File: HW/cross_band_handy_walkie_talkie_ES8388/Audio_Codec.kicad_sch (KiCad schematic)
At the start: 73 parts, among them J3 Screw_Terminal_01x02, J4 Conn_01x06, J5 Screw_Terminal_01x02, J6 AudioJack4_SwitchTR1, J7 SMA, J8 SMA, U5 ES8388, U6 TPA2012D2, U7 SA818S, U8 SA818S

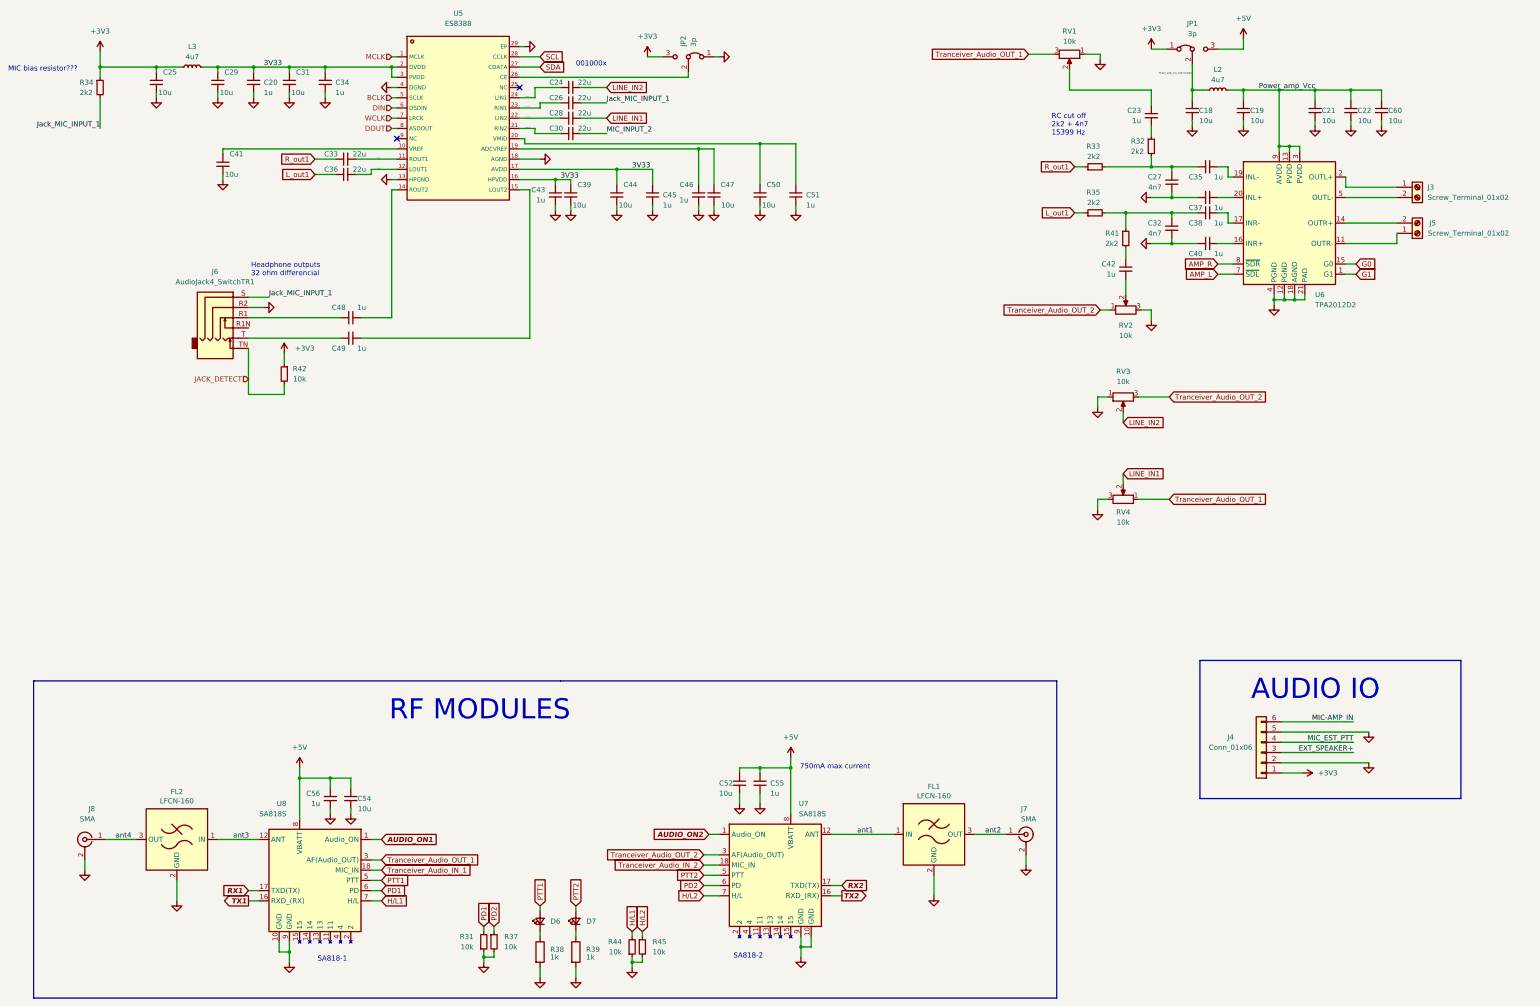
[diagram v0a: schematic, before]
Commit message: r
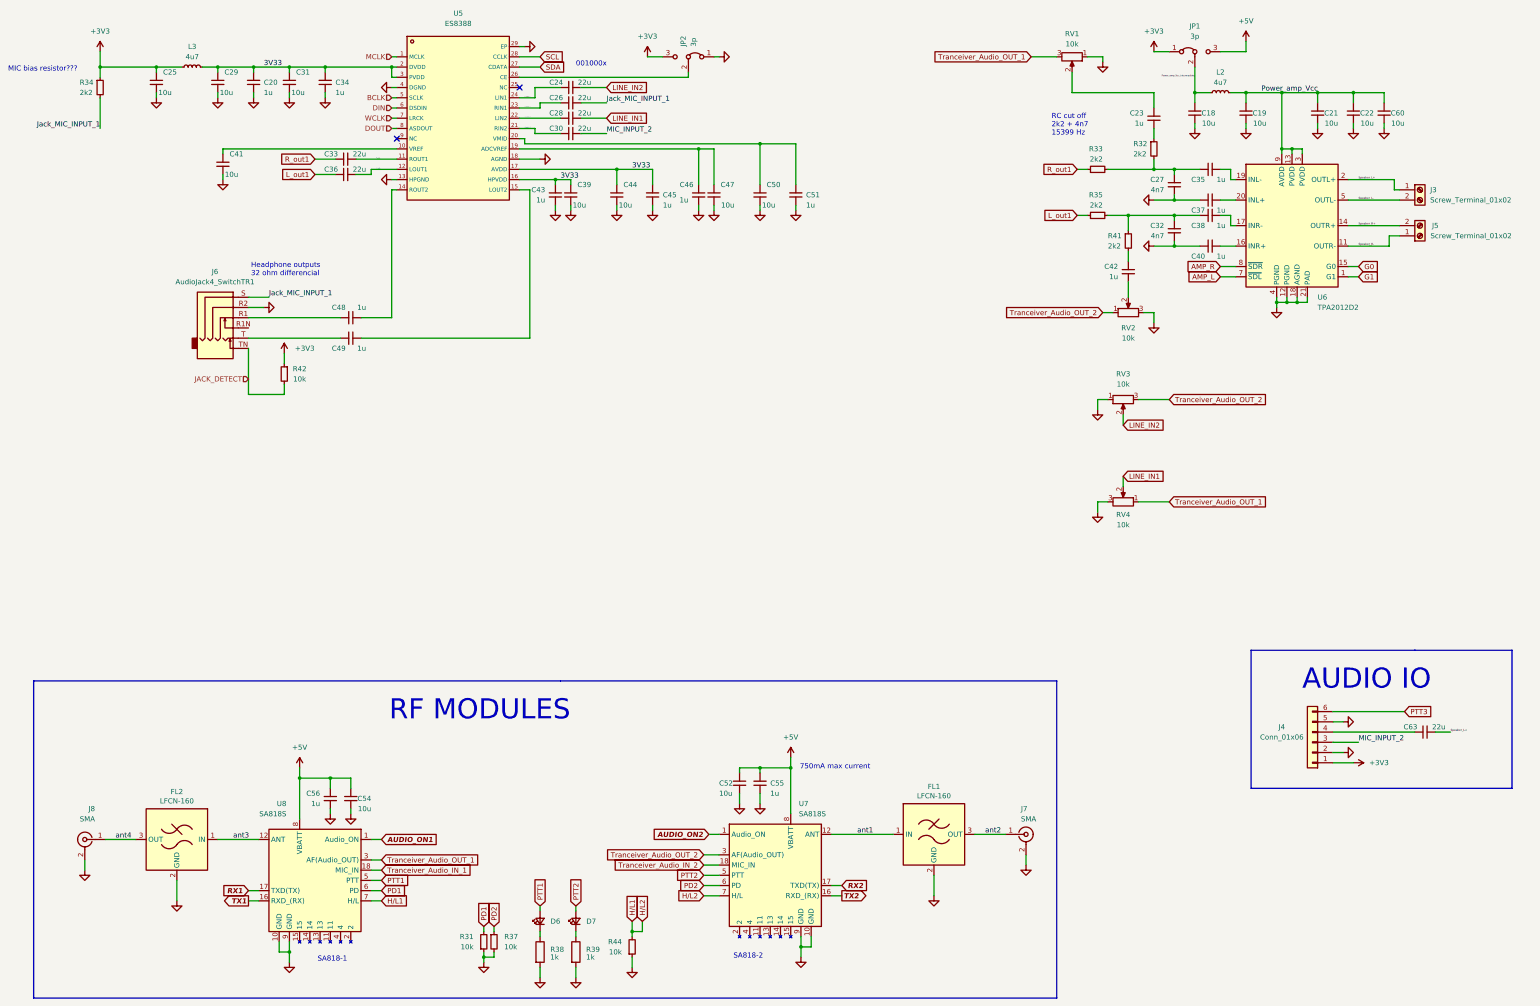
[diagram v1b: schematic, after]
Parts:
- removed R45: 10k, Resistor_SMD:R_0603_1608Metric_Pad0.98x0.95mm_HandSolder, symbol Device:R_Small
- added C63: 22u, Capacitor_SMD:C_0805_2012Metric, symbol Device:C_Small
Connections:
- net EXT_SPEAKER+ is gone; now on net MIC_INPUT_2: J4.3 (Pin_3)
- net H/L2 is gone; now on net H/L1: U7.7 (H/L)
- net Speaker_L+: now reaches J3.1 (Pin_1), U6.2 (OUTL+)
- net Speaker_L+: now also C63.2
- net Speaker_L-: now reaches J3.2 (Pin_2), U6.5 (OUTL-)
- net Speaker_R-: now reaches J5.1 (Pin_1), U6.11 (OUTR-)
- net Speaker_R+: now reaches J5.2 (Pin_2), U6.14 (OUTR+)
- net MIC-AMP_IN renamed PTT3
- net MIC_EST_PTT: no longer names the net of J4.4 (Pin_4)
- net MIC_EST_PTT: now also C63.1
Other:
- moved on the sheet: C18, C19, C21, C22, C23, C27, C32, C35, C37, C38, C40, C42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
